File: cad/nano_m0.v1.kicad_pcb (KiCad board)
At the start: 2 copper layers, 25 parts, among them J1 Conn_01x10, J2 Conn_01x10, J3 USB_B_Micro, J4 SWD, SW1 SW_SPST, SW2 SW_SPST, U1 AP2112K-3.3TRG1, U2 STM32F0706P6, Y1 16MHz

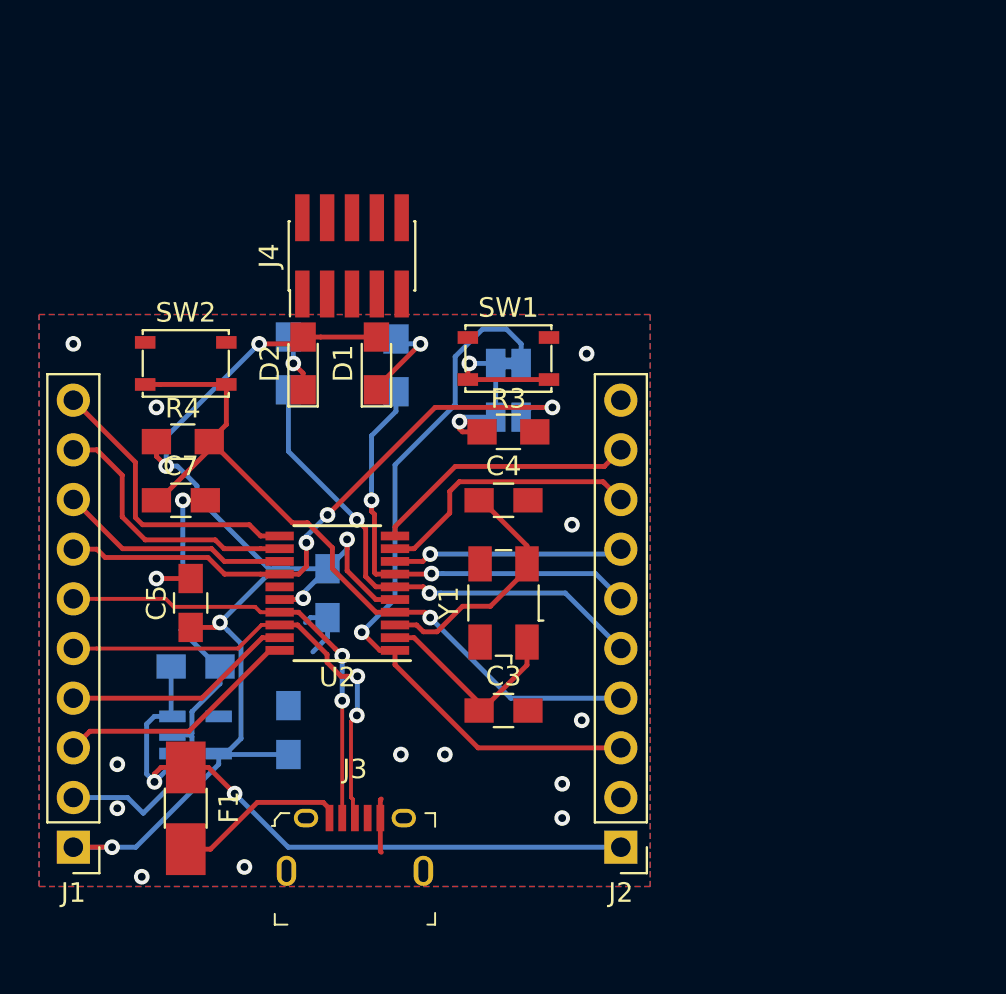
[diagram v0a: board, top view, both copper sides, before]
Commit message: board v2
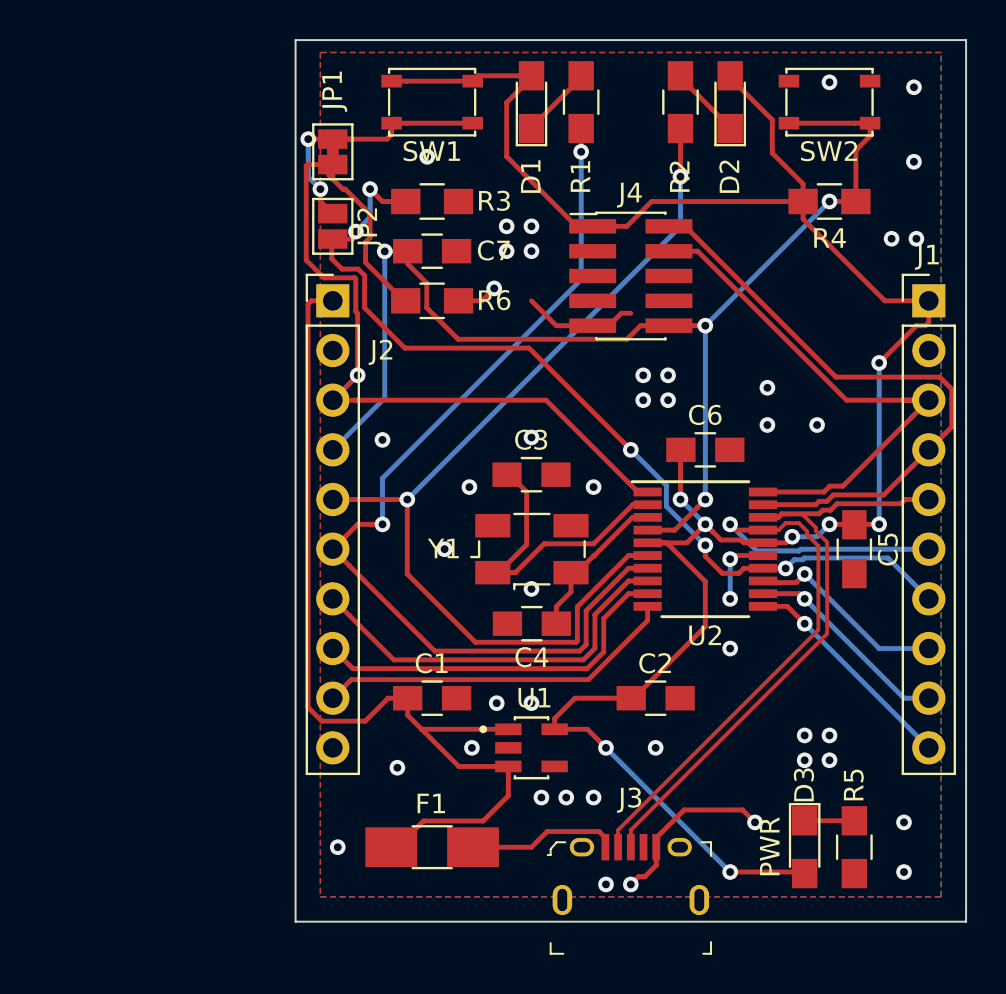
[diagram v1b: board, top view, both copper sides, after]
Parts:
- added D3: PWR, LEDs:LED_0805_HandSoldering, F.Cu at (120.7, 142.2)
- added R5: 80ohm, Resistors_SMD:R_0805_HandSoldering, F.Cu at (123.2, 142.2)
- added R6: 10k, Resistors_SMD:R_0805_HandSoldering, F.Cu at (101.6, 114.3)
- added REF***: OSHW-Logo2_14.6x12mm_SilkScreen, Symbols:OSHW-Logo2_14.6x12mm_SilkScreen, B.Cu at (120.0, 108.6)
- C1, C2, C6, JP1, JP2, R1, R2, U1: moved to F.Cu
- C3, C4: value 22pF -> 15pF
- moved J1 51.9 mm to (127.0, 114.3), turned to 0 degrees
- moved SW2 35.5 mm to (121.9, 104.1)
- moved R4 35.3 mm to (121.9, 109.2)
- moved C5 34.1 mm to (123.2, 127.0), turned to 270 degrees
- moved J2 31.6 mm to (96.5, 114.3), turned to 0 degrees
- moved D2 25.6 mm to (116.8, 104.1)
- moved R2 24.1 mm to (114.3, 104.1)
- moved C6 20.7 mm to (115.6, 121.9), turned to 0 degrees
- moved U2 19.0 mm to (115.6, 127.0), turned to 0 degrees
- moved C2 18.9 mm to (113.0, 134.6), turned to 0 degrees
- moved C7 18.1 mm to (101.6, 111.8)
- moved U1 17.2 mm to (106.7, 137.2)
- moved R1 16.5 mm to (109.2, 104.1)
- moved D1 15.5 mm to (106.7, 104.1)
- moved J4 14.3 mm to (111.8, 113.0), turned to 0 degrees
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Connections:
- R3 pad 1: Net-(JP1-Pad1) -> /PB1
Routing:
- net +3V3: track 65.8 -> 108.4 mm, vias 6 -> 8
- net /PA1: track 23.0 -> 48.5 mm
- net /NRST: track 38.7 -> 62.2 mm, vias 1 -> 4
- net /PA0: track 25.8 -> 49.2 mm
- net /PA13: track 11.8 -> 31.1 mm
- net /PB1: track 31.3 -> 47.4 mm, vias 3 -> 5
- net /PA14: track 12.6 -> 28.1 mm
- net +5V: track 35.1 -> 47.9 mm, vias 2 -> 0
- net /USB_N: track 23.3 -> 35.8 mm, vias 2 -> 1
- net /USB_P: track 23.8 -> 32.6 mm, vias 2 -> 0
- net GND: track 29.6 -> 20.8 mm, vias 15 -> 45
- net /PA2: track 11.8 -> 20.1 mm, vias 1 -> 0
- net /BOOT: track 37.5 -> 43.1 mm
- net /PA3: track 14.0 -> 19.1 mm
- net /OSC_IN: track 10.7 -> 15.7 mm
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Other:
- board outline added: 34.3 x 45.1 mm
- rule pad_to_mask_clearance: 0.2 -> 0
- board text added: "@zklapow"
- board text added: "NANO-M0"
- board text added: "V1"
